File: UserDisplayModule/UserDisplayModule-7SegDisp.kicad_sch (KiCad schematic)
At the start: 15 parts, among them U4 74HC595

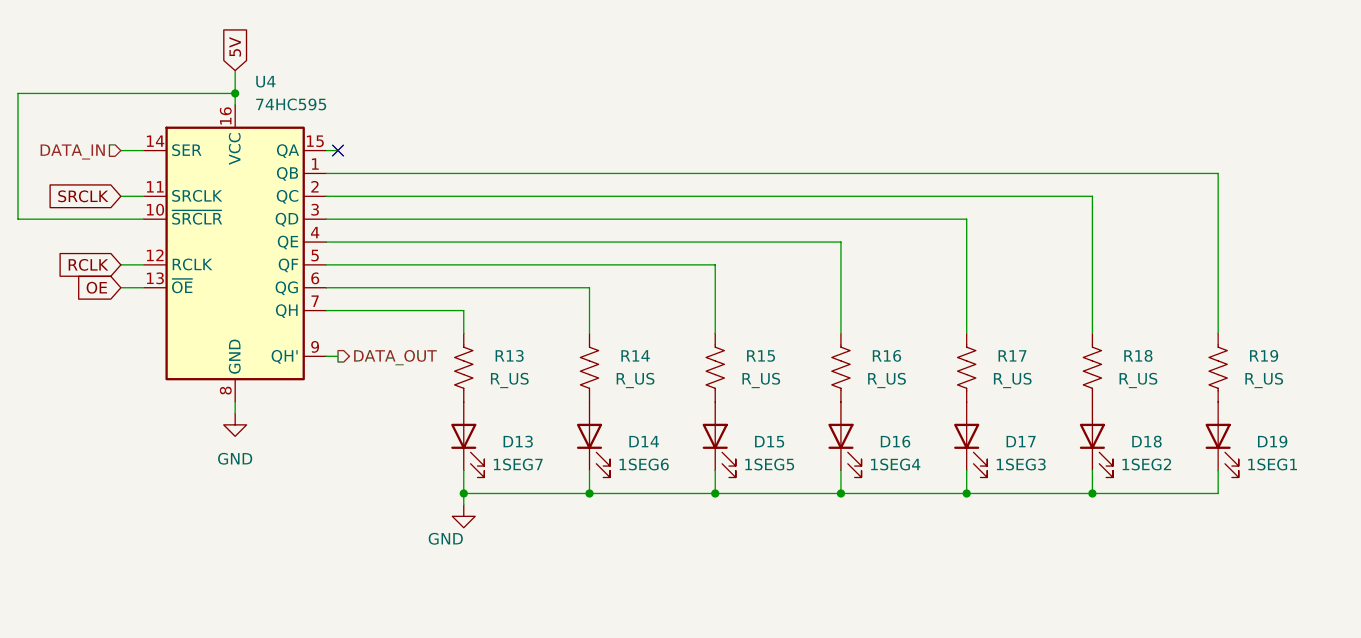
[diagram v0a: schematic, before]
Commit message: doubled LEDs + started PCB
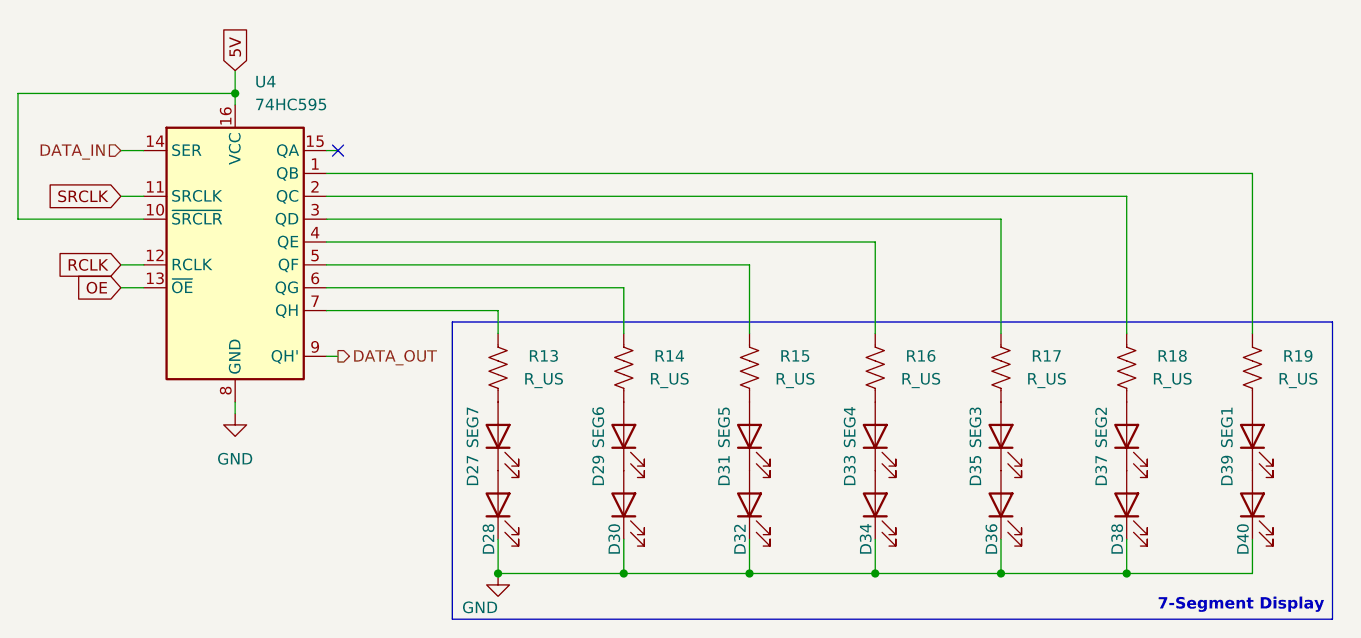
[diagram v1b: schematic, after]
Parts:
- removed D13: 1SEG7, symbol Device:LED
- removed D14: 1SEG6, symbol Device:LED
- removed D15: 1SEG5, symbol Device:LED
- removed D16: 1SEG4, symbol Device:LED
- removed D17: 1SEG3, symbol Device:LED
- removed D18: 1SEG2, symbol Device:LED
- removed D19: 1SEG1, symbol Device:LED
- added D27: SEG7, LED_SMD:LED_0805_2012Metric, symbol Device:LED
- added D28, D30, D32, D34, D36, D38, D40: BAT1, LED_SMD:LED_0805_2012Metric, symbol Device:LED
- added D29: SEG6, LED_SMD:LED_0805_2012Metric, symbol Device:LED
- added D31: SEG5, LED_SMD:LED_0805_2012Metric, symbol Device:LED
- added D33: SEG4, LED_SMD:LED_0805_2012Metric, symbol Device:LED
- added D35: SEG3, LED_SMD:LED_0805_2012Metric, symbol Device:LED
- added D37: SEG2, LED_SMD:LED_0805_2012Metric, symbol Device:LED
- added D39: SEG1, LED_SMD:LED_0805_2012Metric, symbol Device:LED
- R13, R14, R15, R16, R17, R18, R19: footprint (none) -> Resistor_SMD:R_0805_2012Metric
- U4: footprint (none) -> ImportedFootprints:CD74HC595E
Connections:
- net GND: now also D28.1 (K), D30.1 (K), D32.1 (K), D34.1 (K), D36.1 (K), D38.1 (K), D40.1 (K)
- net at R14.2: now also D29.2 (A)
- net at R13.2: now also D27.2 (A)
- net at R15.2: now also D31.2 (A)
- net at R19.2: now also D39.2 (A)
- net at R16.2: now also D33.2 (A)
- net at R18.2: now also D37.2 (A)
- net at R17.2: now also D35.2 (A)
- new net: D29.1 (K), D30.2 (A)
- new net: D31.1 (K), D32.2 (A)
- new net: D37.1 (K), D38.2 (A)
- new net: D27.1 (K), D28.2 (A)
- new net: D39.1 (K), D40.2 (A)
- new net: D35.1 (K), D36.2 (A)
- new net: D33.1 (K), D34.2 (A)
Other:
- note added: "7-Segment Display"
- moved on the sheet: R13, R14, R15, R16, R17, R18, R19
